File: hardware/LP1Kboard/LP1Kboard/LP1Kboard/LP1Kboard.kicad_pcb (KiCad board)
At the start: 2 copper layers, 124.5 x 96.5 mm, 30 parts, among them J1 Conn_02x05_Odd_Even, J6 Conn_01x03_Male, U1 LTC3406ES5, U2 AT25SF081-SSHD-X, U3 ICE40LP1K-CM36

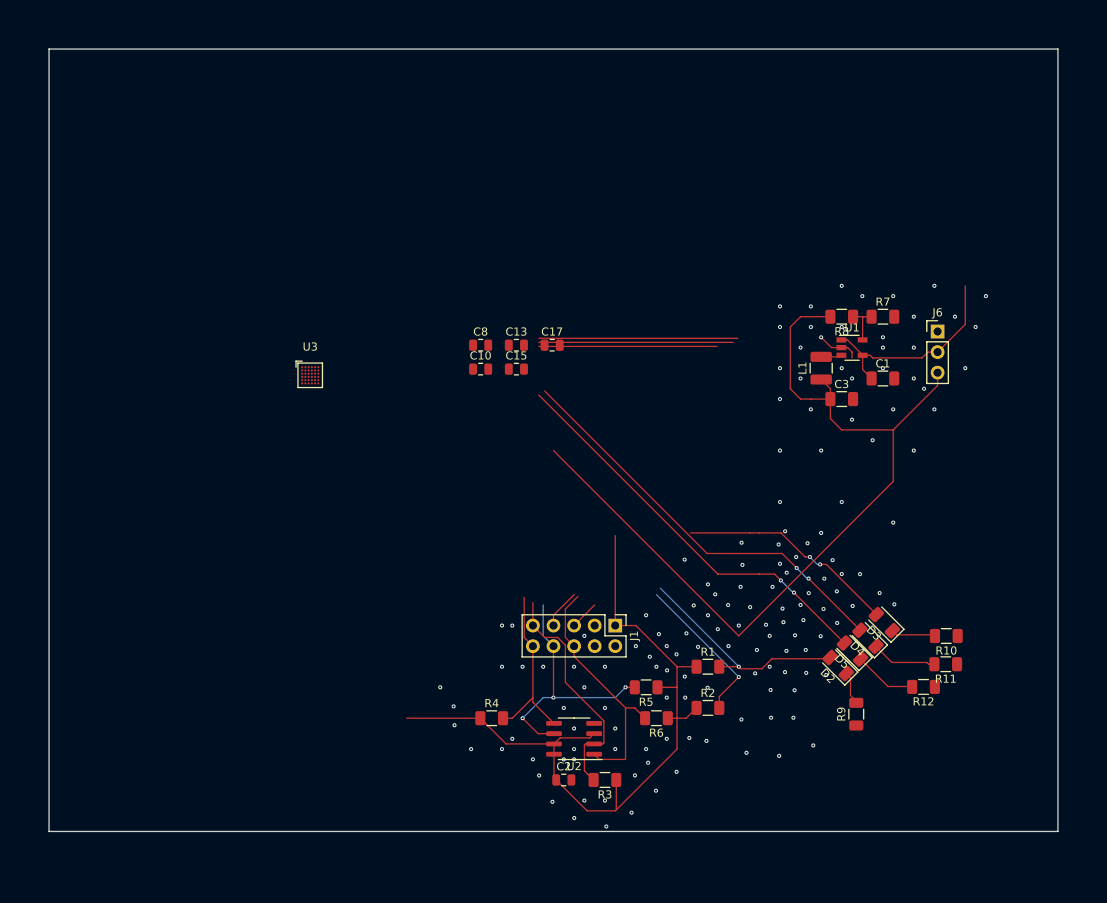
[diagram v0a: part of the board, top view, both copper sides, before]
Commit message: LP1K + HX1Kcap boards
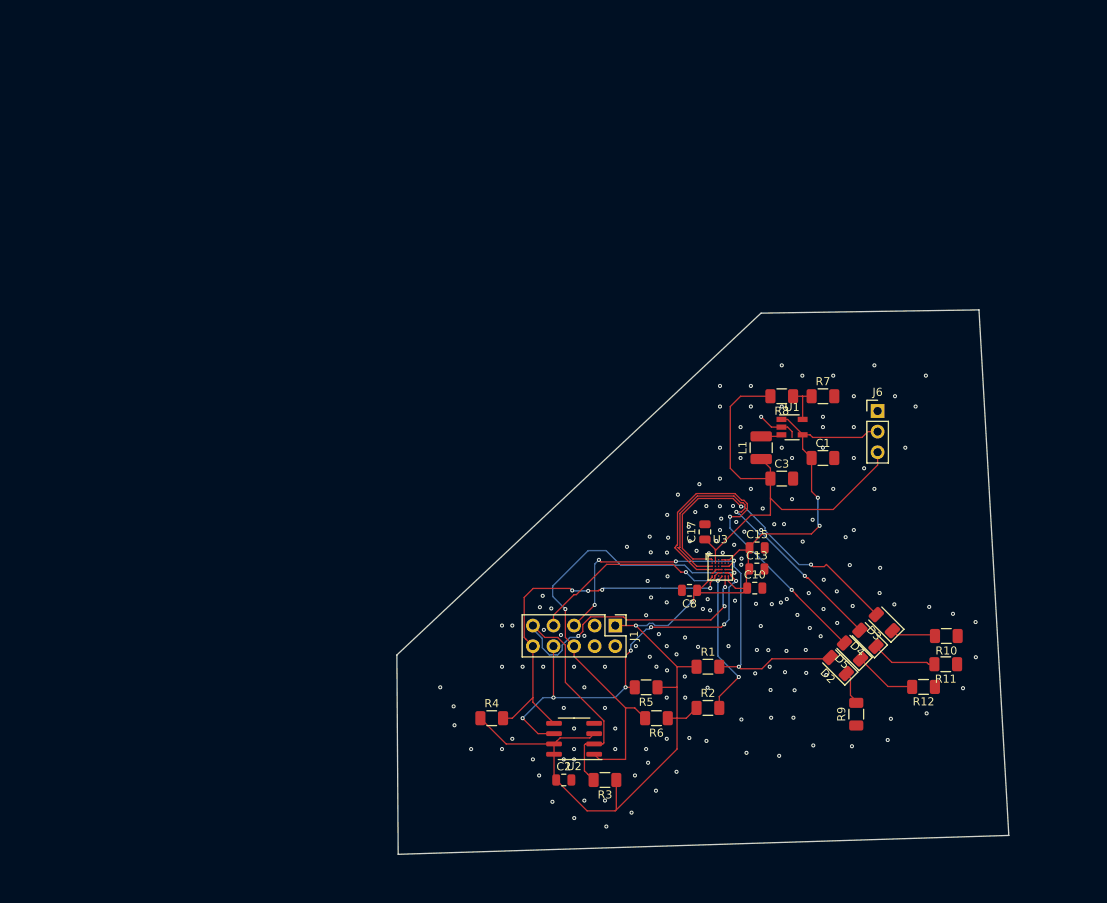
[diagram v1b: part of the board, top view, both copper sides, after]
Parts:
- U3: footprint Package_CSP:WLCSP-36_2.82x2.67mm_Layout6x6_P0.4mm -> kifootp:ice40-CM36-WLCSP-36_2.82x2.67mm_Layout6x6_P0.4mm
- moved U3 55.9 mm to (166.6, 107.2)
- moved C10 43.3 mm to (170.9, 109.7)
- moved C13 40.5 mm to (171.1, 107.3)
- moved C8 39.7 mm to (162.8, 110.0), turned to 180 degrees
- moved C15 37.0 mm to (171.2, 104.7)
- moved C17 29.8 mm to (164.7, 102.7), turned to 90 degrees
- moved C1 12.3 mm to (179.3, 93.6)
- moved C3 12.3 mm to (174.2, 96.2)
- moved J6 12.3 mm to (186.0, 87.8)
- moved L1 12.3 mm to (171.7, 92.4)
- moved R7 12.3 mm to (179.3, 86.0)
- moved R8 12.3 mm to (174.2, 86.0)
- moved U1 12.3 mm to (175.5, 89.8)
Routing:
- net +1V2: track 107.1 -> 55.6 mm
- net SPI_IN: track 29.2 -> 60.0 mm, vias 0 -> 3
- net SPI_CS: track 30.9 -> 58.8 mm, vias 0 -> 2
- net SPI_OUT: track 21.8 -> 48.2 mm, vias 0 -> 4
- net IO65: track 24.5 -> 0.00 mm
- net CDONE: track 31.4 -> 55.7 mm, vias 1 -> 5
- net IO64: track 24.0 -> 0.00 mm
- net IO63: track 22.0 -> 0.00 mm
- net SPI_SCK: track 32.0 -> 52.4 mm, vias 3 -> 7
- net +3V3: track 118.7 -> 138.2 mm, vias 0 -> 4
- net CRESET: track 24.0 -> 43.5 mm, vias 1 -> 3
- net IO1: track 27.0 -> 39.5 mm
- net IO2: track 51.2 -> 42.0 mm
- net IO3: track 50.5 -> 45.4 mm
- net GND: track 5.28 -> 6.89 mm, vias 147 -> 175
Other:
- board size 124.5 x 96.5 mm -> 75.5 x 67.2 mm
